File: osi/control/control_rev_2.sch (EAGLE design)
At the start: 5 parts

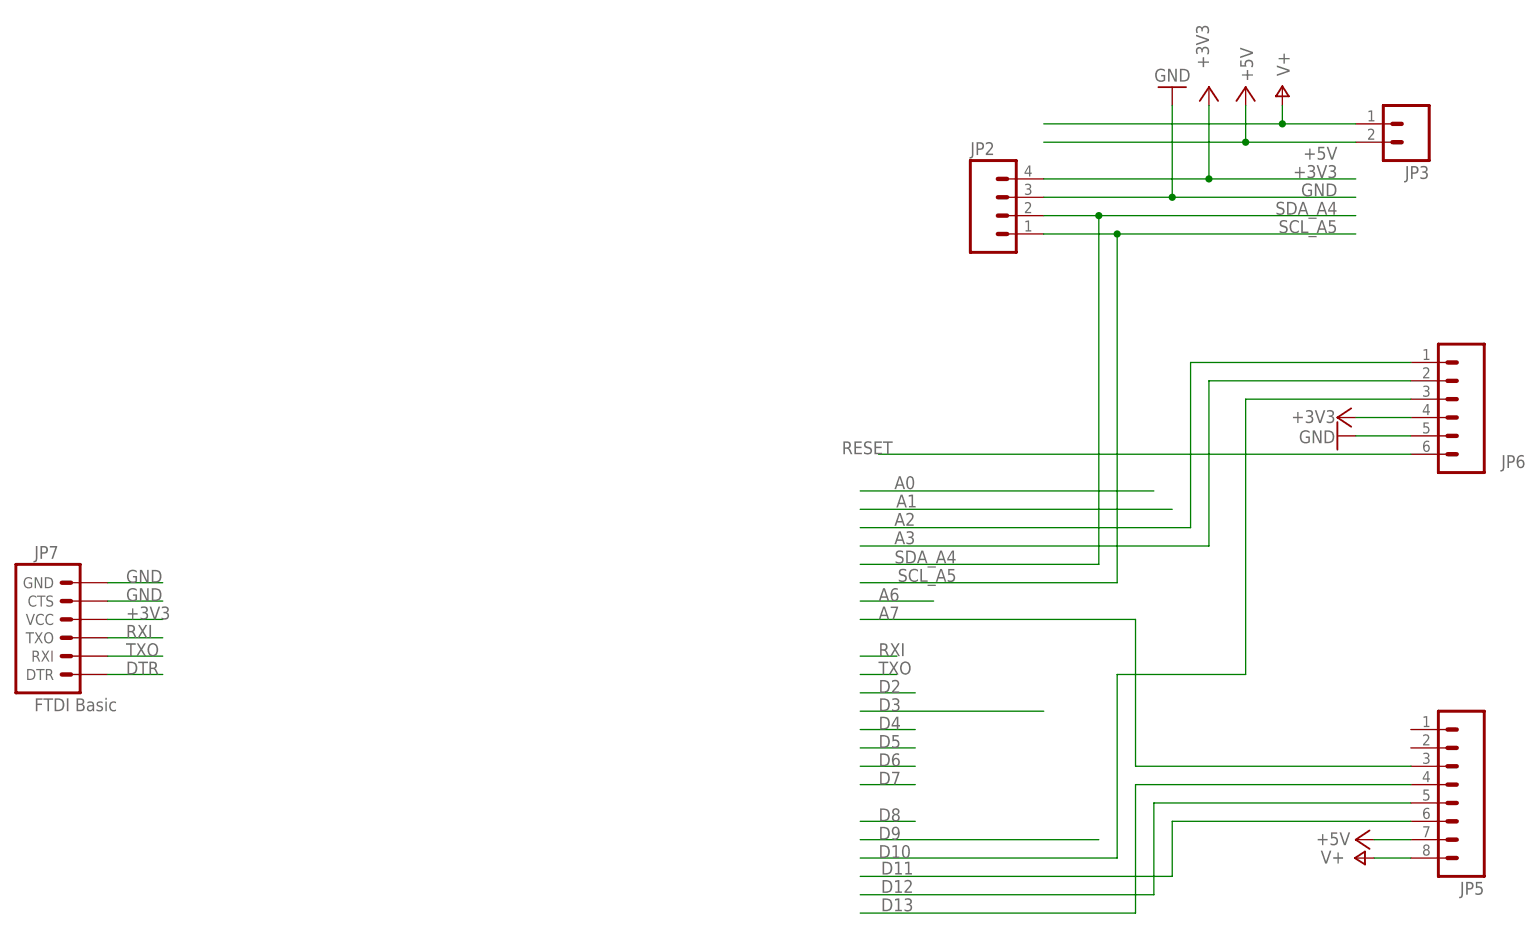
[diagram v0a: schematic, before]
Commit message: layout changes
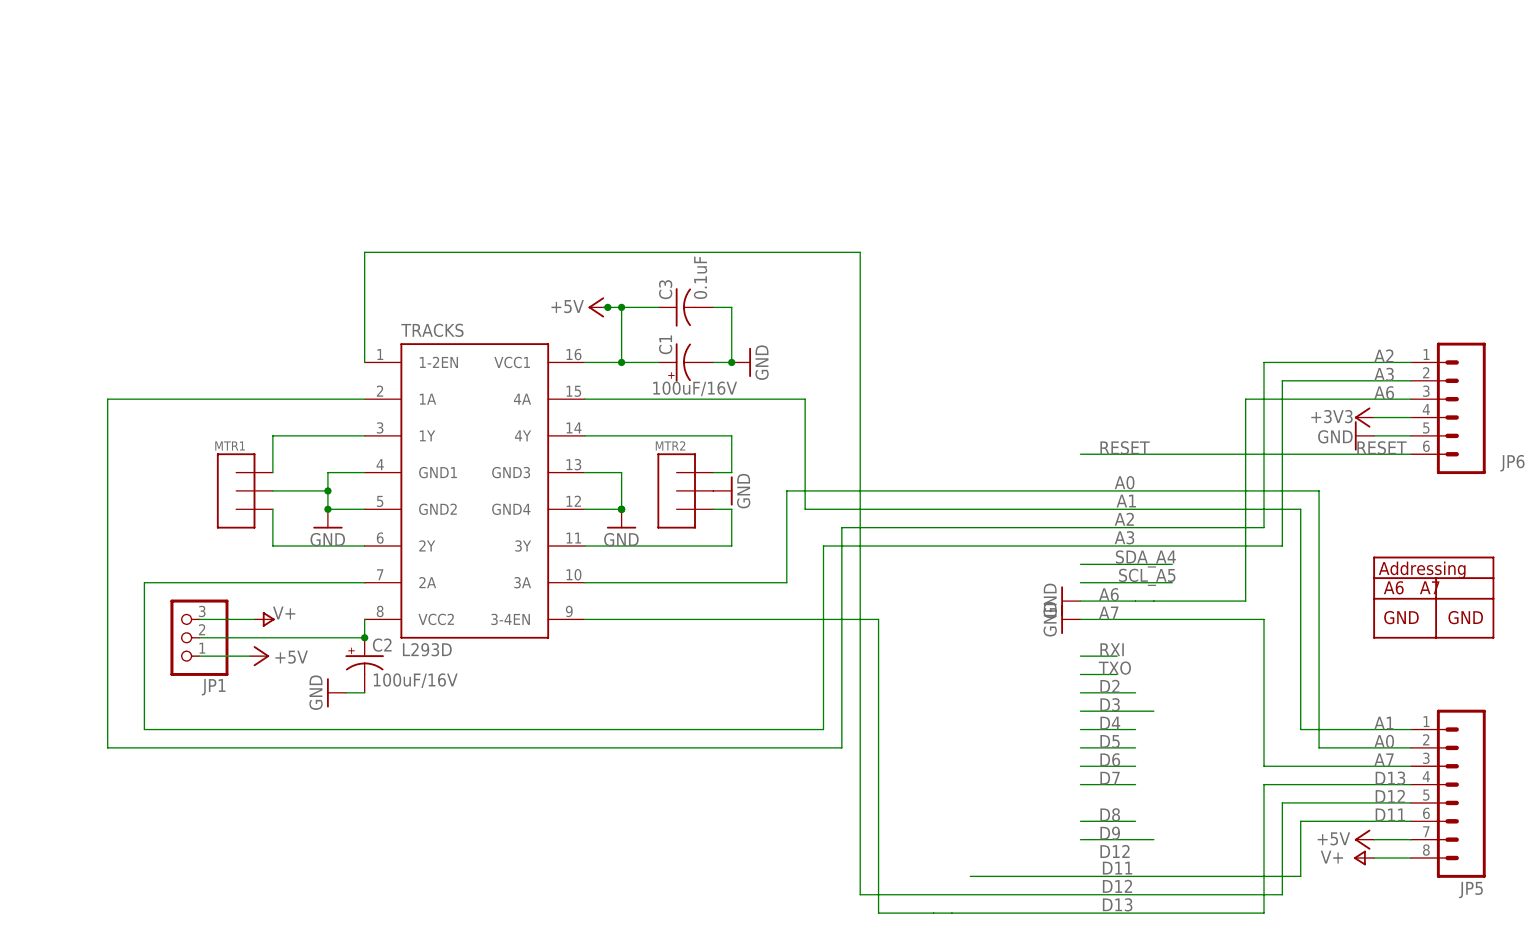
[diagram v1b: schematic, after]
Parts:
- removed JP2: (no value), SparkFun_mod:M04PTH
- removed JP3: (no value), SparkFun_mod:M02PTH
- removed JP7: FTDI Basic, SparkFun:ARDUINO_SERIAL_PROGRAMPTH
- added C1, C2: 100uF/16V, rcl-ez:CPOL-USE2.5-6
- added C3: 0.1uF, rcl-ez:C-US025-025X050
- added JP1: (no value), adafruit_mod:PINHD-1X3
- added MTR1, MTR2: TERMINAL, _my-parts:TERMINAL
- added TRACKS: L293D, texas:L293E
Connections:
- net D10 renamed A6
- removed net DTR: JP7.DTR
- removed net RXI: JP7.TXO
- removed net SCL_A5: JP2.1
- removed net SDA_A4: JP2.2
- removed net TXO: JP7.RXI
- new net A0: JP5.2, TRACKS.3A
- new net A1: JP5.1, TRACKS.4A
- new net N$1: MTR1.P$1, TRACKS.1Y
- new net N$2: MTR2.P$1, TRACKS.4Y
- new net N$3: MTR1.P$3, TRACKS.2Y
- new net N$4: MTR2.P$3, TRACKS.3Y
- new net N$8: C2.+, JP1.2, TRACKS.VCC2
- net +3V3: no longer JP2.4, JP7.VCC
- net +5V: now also C1.+, C3.1, JP1.1, TRACKS.VCC1; no longer JP3.2
- net A2: now also TRACKS.1A
- net A3: now also TRACKS.2A
- net D12: now also TRACKS.1-2EN
- net D13: now also TRACKS.3-4EN
- net GND: now also C1.-, C2.-, C3.2, MTR1.P$2, MTR2.P$2, TRACKS.GND1, TRACKS.GND2, TRACKS.GND3, TRACKS.GND4; no longer JP2.3, JP7.CTS, JP7.GND
- net V+: now also JP1.3; no longer JP3.1
